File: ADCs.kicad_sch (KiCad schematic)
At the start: 21 parts, among them J10 Conn_01x03, J11 Conn_01x03, J12 Conn_01x03, J14 Conn_01x03, J15 Conn_01x03, J16 Conn_01x03, J3 Conn_01x03, J4 Conn_01x03, J5 Conn_01x03, J7 Conn_01x03, J8 Conn_01x03, J9 Conn_01x03, U13 TCA9517ADGK, U3 ADS7828, U4 ADS7828

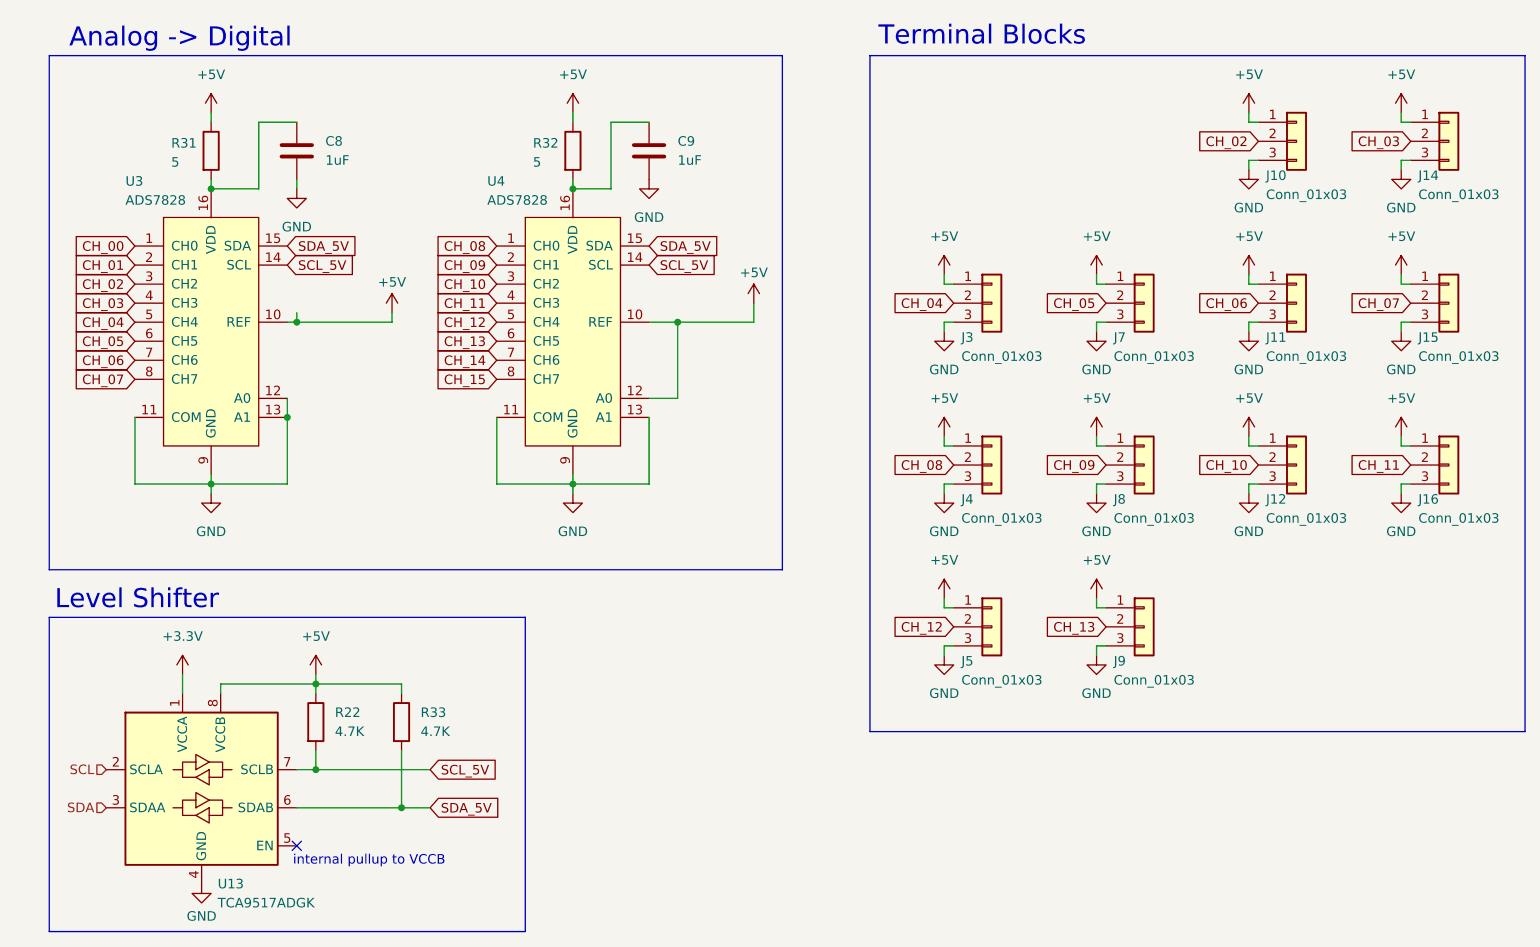
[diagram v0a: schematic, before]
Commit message: Initial pass at finding Mouser part numbers
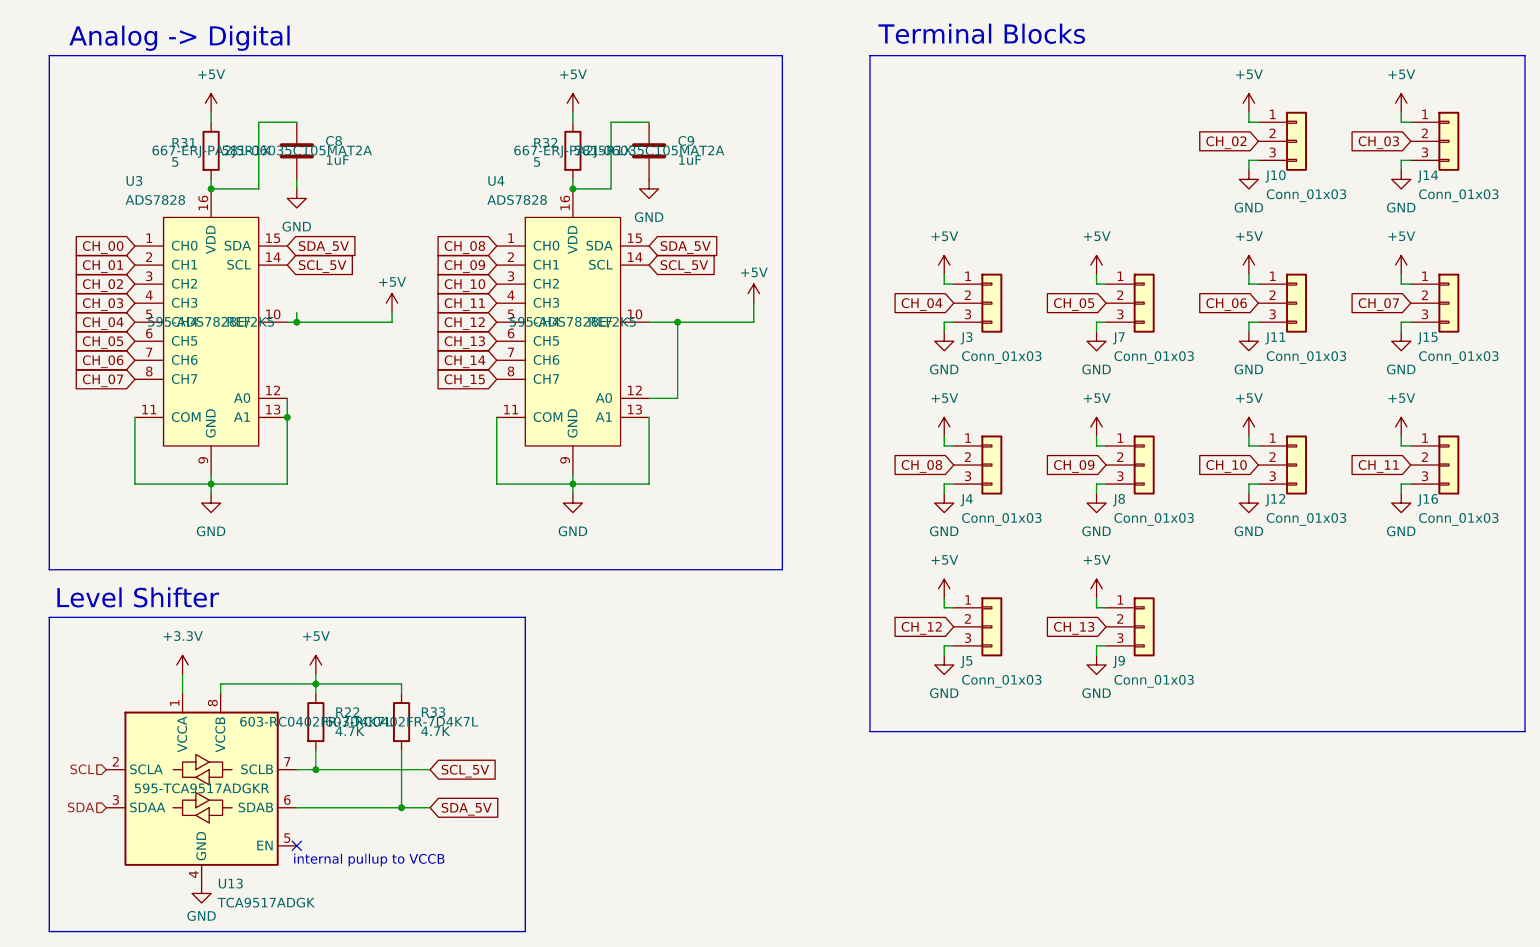
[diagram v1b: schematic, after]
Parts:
- C8, C9: Mouser Part Number  (none) -> 581-06035C105MAT2A
- R22, R33: Mouser Part Number  (none) -> 603-RC0402FR-7D4K7L
- R31, R32: Mouser Part Number  (none) -> 667-ERJ-PA2J5R1X
- U13: Mouser Part Number  (none) -> 595-TCA9517ADGKR
- U3, U4: Mouser Part Number  (none) -> 595-ADS7828E/2K5
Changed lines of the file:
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@@
 			)
 		)
+		(property "Mouser Part Number " ""
+			(at 220.98 113.03 0)
+			(effects
+				(font
+					(size 1.27 1.27)
+				)
+			)
+		)
 		(pin "1"
 		)
@@
 			)
 		)
+		(property "Mouser Part Number " ""
+			(at 220.98 69.85 0)
+			(effects
+				(font
+					(size 1.27 1.27)
+				)
+			)
+		)
 		(pin "1"
 		)
@@
 			)
 		)
+		(property "Mouser Part Number " "595-ADS7828E/2K5 "
+			(at 124.46 93.98 0)
+			(effects
+				(font
+					(size 1.27 1.27)
+				)
+			)
+		)
 		(pin "3"
 		)
@@
 			)
 		)
+		(property "Mouser Part Number " ""
+			(at 200.66 91.44 0)
+			(effects
+				(font
+					(size 1.27 1.27)
+				)
+			)
+		)
 		(pin "1"
 		)
@@
 			)
 		)
+		(property "Mouser Part Number " "595-ADS7828E/2K5 "
+			(at 76.2 93.98 0)
+			(effects
+				(font
+					(size 1.27 1.27)
+				)
+			)
+		)
 		(pin "3"
 		)
@@
 			)
 		)
+		(property "Mouser Part Number " "581-06035C105MAT2A "
+			(at 87.63 71.12 0)
+			(effects
+				(font
+					(size 1.27 1.27)
+				)
+			)
+		)
 		(pin "1"
 		)
@@
 			)
 		)
+		(property "Mouser Part Number " ""
+			(at 200.66 134.62 0)
+			(effects
+				(font
+					(size 1.27 1.27)
+				)
+			)
+		)
 		(pin "1"
 		)
@@
 			)
 		)
+		(property "Mouser Part Number " ""
+			(at 180.34 91.44 0)
+			(effects
+				(font
+					(size 1.27 1.27)
+				)
+			)
+		)
 		(pin "1"
 		)
@@
 			)
 		)
+		(property "Mouser Part Number " ""
+			(at 241.3 91.44 0)
+			(effects
+				(font
+					(size 1.27 1.27)
+				)
+			)
+		)
 		(pin "1"
 		)
@@
 			)
 		)
+		(property "Mouser Part Number " "603-RC0402FR-7D4K7L "
+			(at 90.17 147.32 0)
+			(effects
+				(font
+					(size 1.27 1.27)
+				)
+			)
+		)
 		(pin "1"
 		)
@@
 			)
 		)
+		(property "Mouser Part Number " ""
+			(at 220.98 91.44 0)
+			(effects
+				(font
+					(size 1.27 1.27)
+				)
+			)
+		)
 		(pin "1"
 		)
@@
 			)
 		)
+		(property "Mouser Part Number " ""
+			(at 180.34 113.03 0)
+			(effects
+				(font
+					(size 1.27 1.27)
+				)
+			)
+		)
 		(pin "1"
 		)
@@
 			)
 		)
+		(property "Mouser Part Number " "603-RC0402FR-7D4K7L "
+			(at 101.6 147.32 0)
+			(effects
+				(font
+					(size 1.27 1.27)
+				)
+			)
+		)
 		(pin "1"
 		)
@@
 			)
 		)
+		(property "Mouser Part Number " "667-ERJ-PA2J5R1X "
+			(at 124.46 71.12 0)
+			(effects
+				(font
+					(size 1.27 1.27)
+				)
+			)
+		)
 		(pin "1"
 		)
@@
 			)
 		)
+		(property "Mouser Part Number " "667-ERJ-PA2J5R1X "
+			(at 76.2 71.12 0)
+			(effects
+				(font
+					(size 1.27 1.27)
+				)
+			)
+		)
 		(pin "1"
 		)
@@
 			)
 		)
+		(property "Mouser Part Number " ""
+			(at 241.3 69.85 0)
+			(effects
+				(font
+					(size 1.27 1.27)
+				)
+			)
+		)
 		(pin "1"
 		)
@@
 			)
 		)
+		(property "Mouser Part Number " "595-TCA9517ADGKR "
+			(at 74.93 156.21 0)
+			(effects
+				(font
+					(size 1.27 1.27)
+				)
+			)
+		)
 		(pin "7"
 		)
@@
 			)
 		)
+		(property "Mouser Part Number " "581-06035C105MAT2A "
+			(at 134.62 71.12 0)
+			(effects
+				(font
+					(size 1.27 1.27)
+				)
+			)
+		)
 		(pin "1"
 		)
@@
 			)
 		)
+		(property "Mouser Part Number " ""
+			(at 200.66 113.03 0)
+			(effects
+				(font
+					(size 1.27 1.27)
+				)
+			)
+		)
 		(pin "1"
 		)
@@
 			)
 		)
+		(property "Mouser Part Number " ""
+			(at 241.3 113.03 0)
+			(effects
+				(font
+					(size 1.27 1.27)
+				)
+			)
+		)
 		(pin "1"
 		)
@@
 			)
 		)
+		(property "Mouser Part Number " ""
+			(at 180.34 134.62 0)
+			(effects
+				(font
+					(size 1.27 1.27)
+				)
+			)
+		)
